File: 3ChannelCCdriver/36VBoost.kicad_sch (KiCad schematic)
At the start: 9 parts, among them U5 XL6019

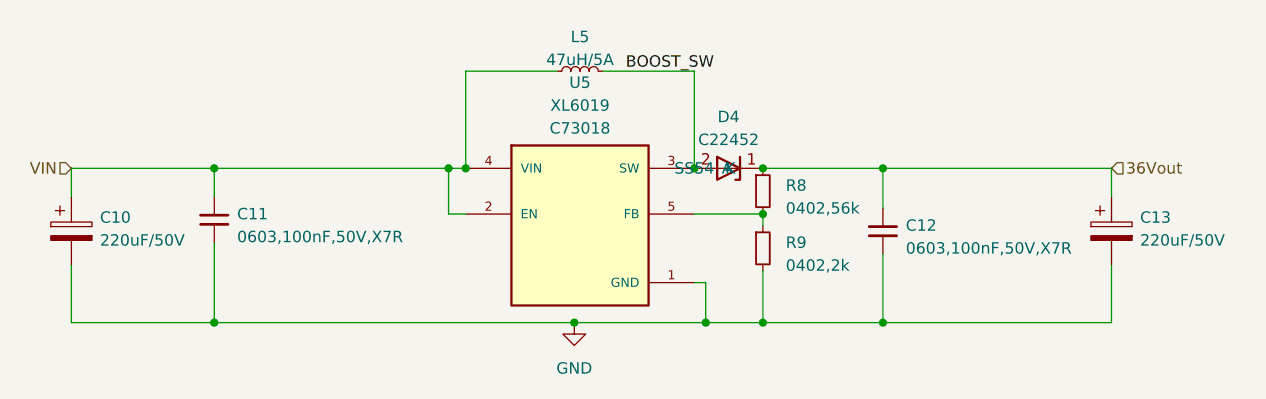
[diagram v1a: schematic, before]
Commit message: neat-ified schematics
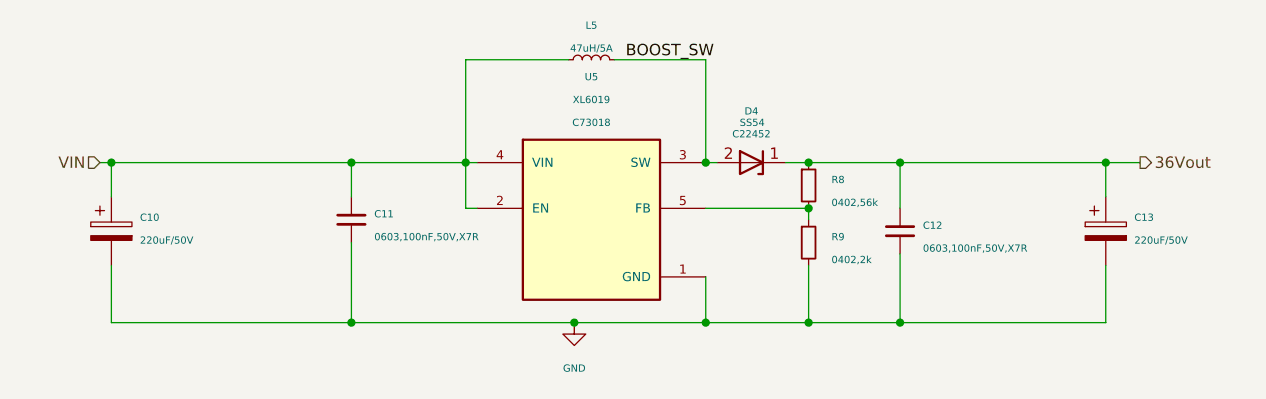
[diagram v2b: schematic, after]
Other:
- moved on the sheet: C10, C11, C12, C13, L5, R8, R9, U5
